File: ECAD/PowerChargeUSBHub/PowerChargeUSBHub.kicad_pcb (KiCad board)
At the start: 2 copper layers, 74 x 30 mm, 15 parts, among them J1 USB_A, J2 USB_A, J3 USB_A, J4 USB_C_Receptacle_PowerOnly_6P

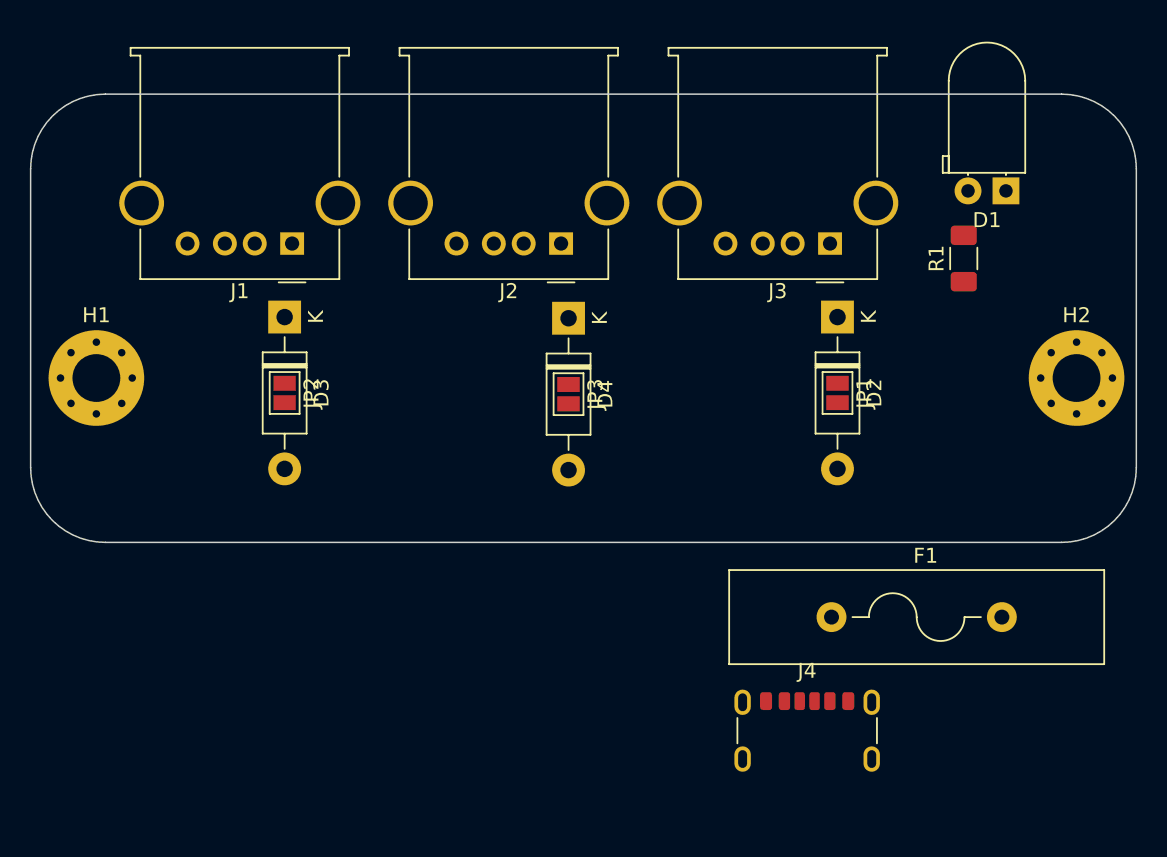
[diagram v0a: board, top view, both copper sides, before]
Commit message: Create Dock
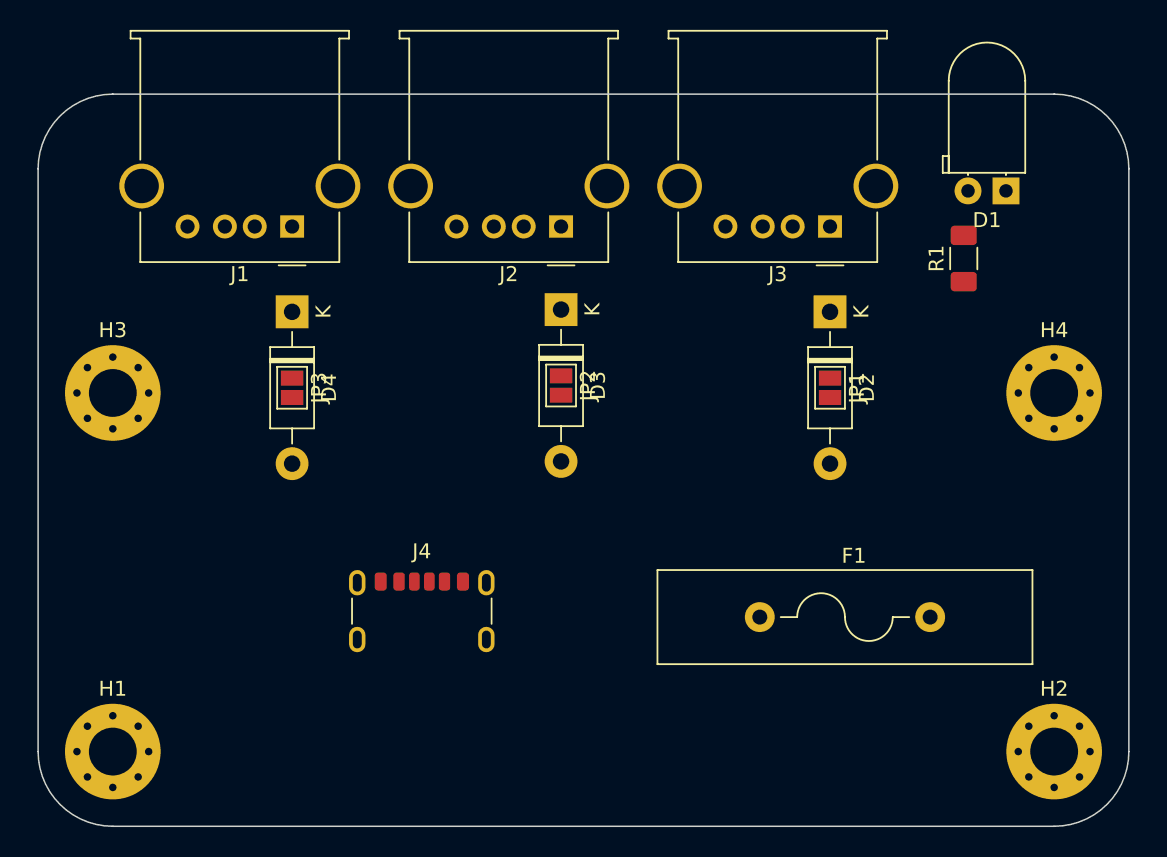
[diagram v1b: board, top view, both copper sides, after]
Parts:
- added H3: M3, MountingHole:MountingHole_3.2mm_M3_Pad_Via, F.Cu at (160.5, 80.0)
- added H4: M3, MountingHole:MountingHole_3.2mm_M3_Pad_Via, F.Cu at (223.5, 80.0)
- moved J4 27.0 mm to (181.2, 95.7)
- moved H2 25.0 mm to (223.5, 104.0)
- moved H1 25.0 mm to (160.5, 104.0)
- moved D3 18.5 mm to (190.5, 74.4)
- moved JP2 18.5 mm to (190.5, 79.5)
- moved D4 18.5 mm to (172.5, 74.6)
- moved JP3 18.5 mm to (172.5, 79.7)
- moved F1 4.80 mm to (203.8, 95.0)
- moved J1 1.14 mm to (172.5, 68.9)
- moved J2 1.14 mm to (190.5, 68.9)
- moved J3 1.14 mm to (208.5, 68.9)
- moved D2 0.61 mm to (208.5, 74.6)
- moved JP1 0.61 mm to (208.5, 79.7)
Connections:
- J1 pad 1: Net-(D3-K) -> Net-(D4-K)
- J2 pad 1: Net-(D4-K) -> Net-(D3-K)
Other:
- board size 74 x 30 mm -> 73 x 49 mm
